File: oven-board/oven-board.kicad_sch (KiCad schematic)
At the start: 30 parts, among them J1 temp_sensor, J2 heating element, J3 wall outlet, J4 12V Power Supply, K1 G2RL-1A-E, SW1 SW_Push, SW2 SW_Push, SW3 SW_Push, SW4 SW_Push, SW5 SW_Push, U1 MCP6004, U2 MCP6L04-xST, U3 NUCLEO-L432KC, U4 SZNUD3124LT1G, U5 NHD-C0220BIZ

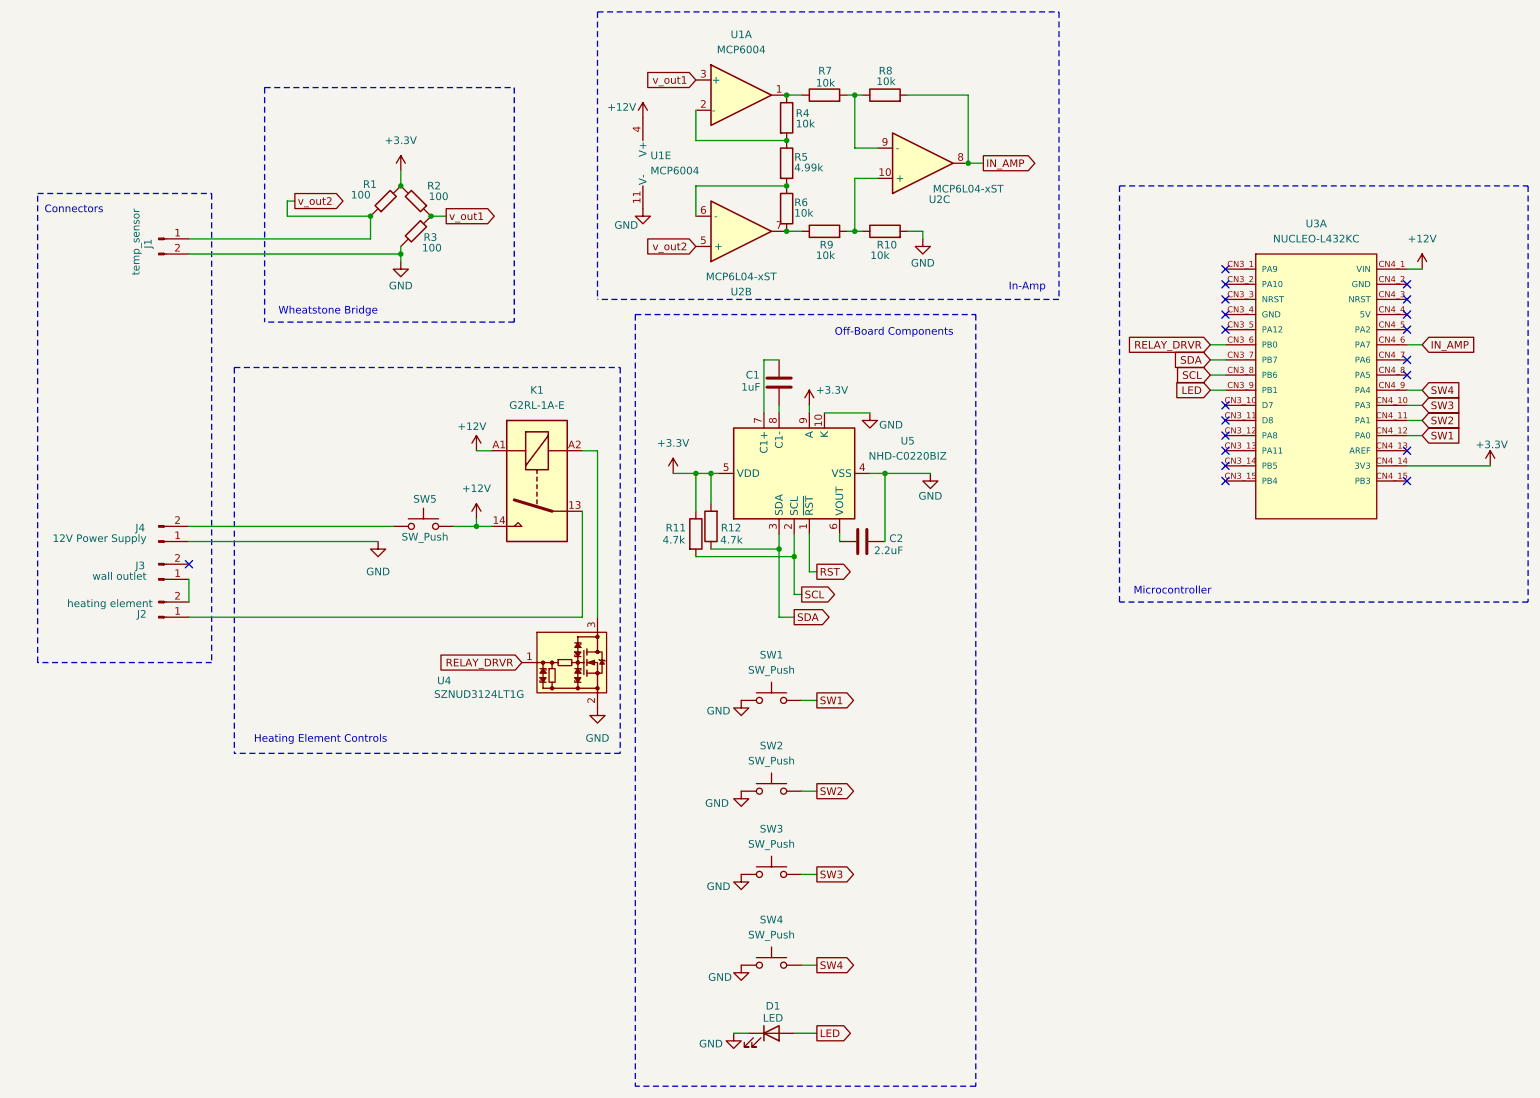
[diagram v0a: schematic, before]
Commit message: OvenBoard Schematic Rev 1.1
Made a few changes to fix schematic, more changes still left
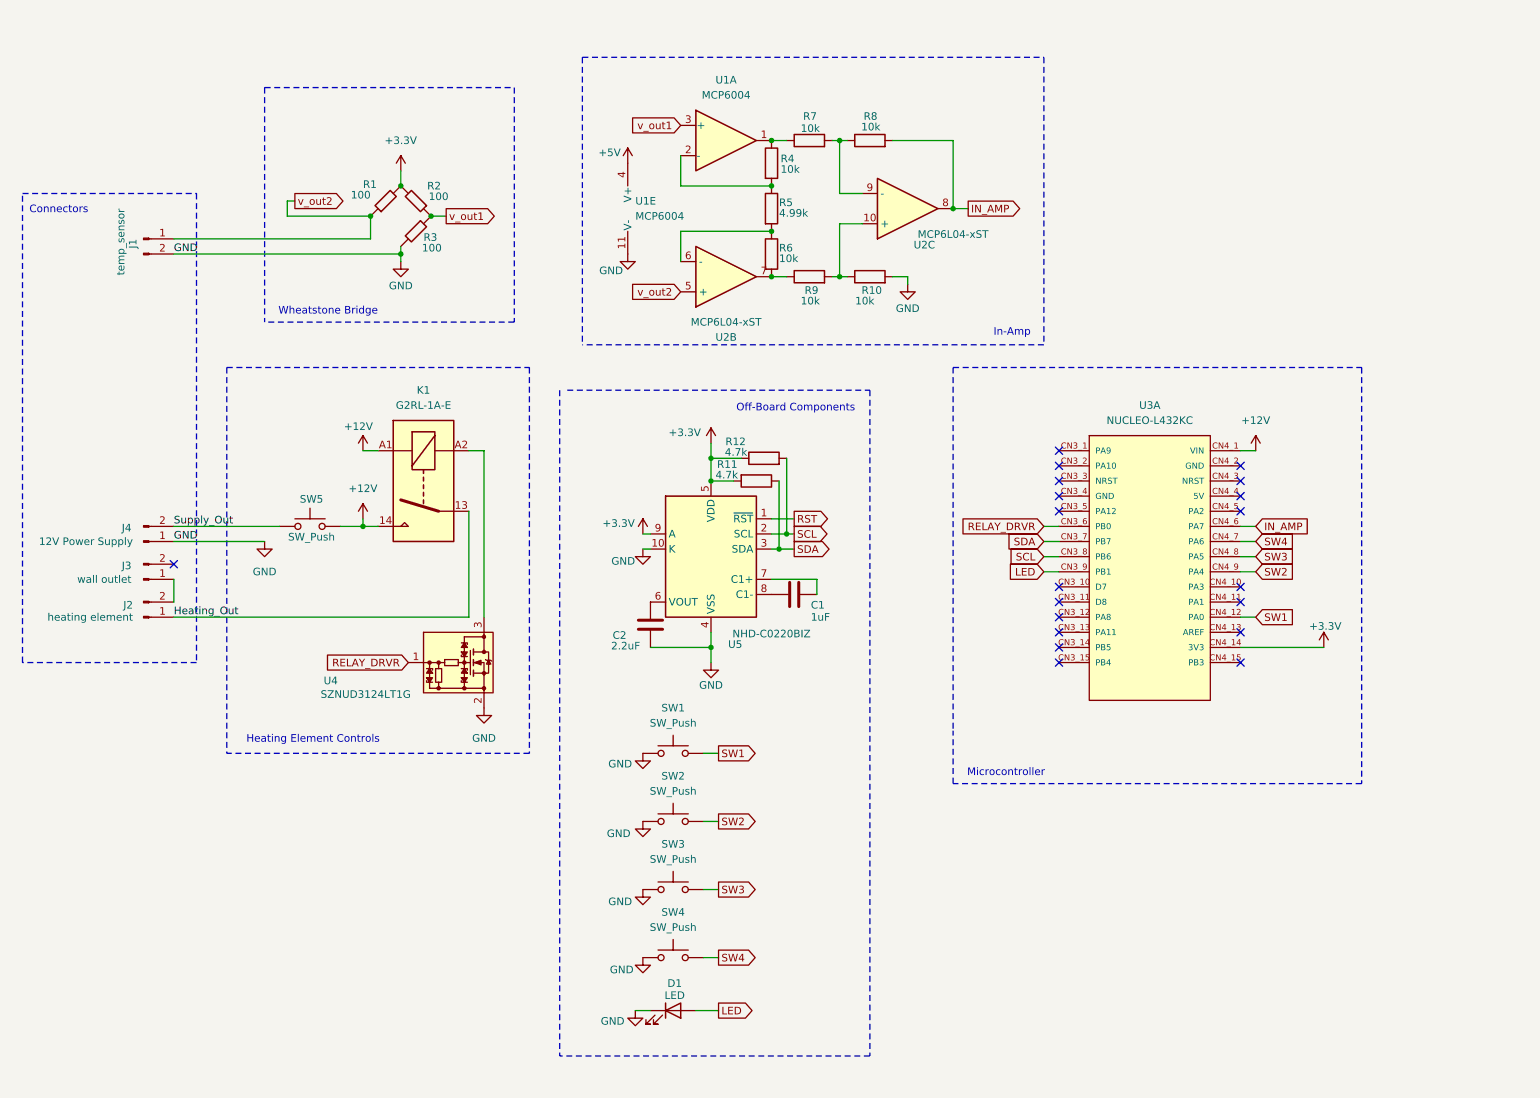
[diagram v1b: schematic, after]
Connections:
- net +12V: no longer U1.4 (V+)
- net +3.3V: now also R11.2, R12.1; no longer R11.1, R12.2
- net SCL: now also R12.2; no longer R11.2
- net SDA: now also R11.1; no longer R12.1
- net SW2: now also U3.CN4_9 (PA4); no longer U3.CN4_11 (PA1)
- net SW3: now also U3.CN4_8 (PA5); no longer U3.CN4_10 (PA3)
- net SW4: now also U3.CN4_7 (PA6); no longer U3.CN4_9 (PA4)
- net Supply_Out: now reaches J4.2 (Pin_2), SW5.2
- net Heating_Out: now reaches J2.1 (Pin_1), K1.13
- new net +5V: U1.4 (V+)
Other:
- moved on the sheet: C1, C2, D1, J1, J2, J3, J4, K1, R10, R11, R12, R4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
